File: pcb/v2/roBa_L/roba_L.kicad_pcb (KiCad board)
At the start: 2 copper layers, 123.9 x 94.5 mm, 56 parts, among them J1 Conn_01x01-Connector_Generic, J2 Conn_01x01-Connector_Generic, J3 Conn_01x01-Connector_Generic, J4 Conn_01x01-Connector_Generic, J5 Conn_01x01-Connector_Generic, J6 Conn_01x01-Connector_Generic, J7 Conn_01x01-Connector_Generic, SW1 SW_PUSH, SW10 SW_PUSH, SW11 SW_PUSH, SW12 SW_PUSH, SW13 SW_PUSH, SW14 SW_PUSH, SW15 SW_PUSH, SW16 SW_PUSH, SW17 SW_PUSH, SW18 SW_PUSH, SW19 SW_PUSH, SW2 SW_PUSH, SW20 SW_PUSH, SW21 RotaryEncoder_Switch, SW22 SW_PUSH, SW23 SW_PUSH, SW24 SW_SPDT, SW3 SW_PUSH, SW4 SW_PUSH, SW5 SW_PUSH, SW6 SW_PUSH, SW7 SW_PUSH, SW8 SW_PUSH, SW9 SW_PUSH

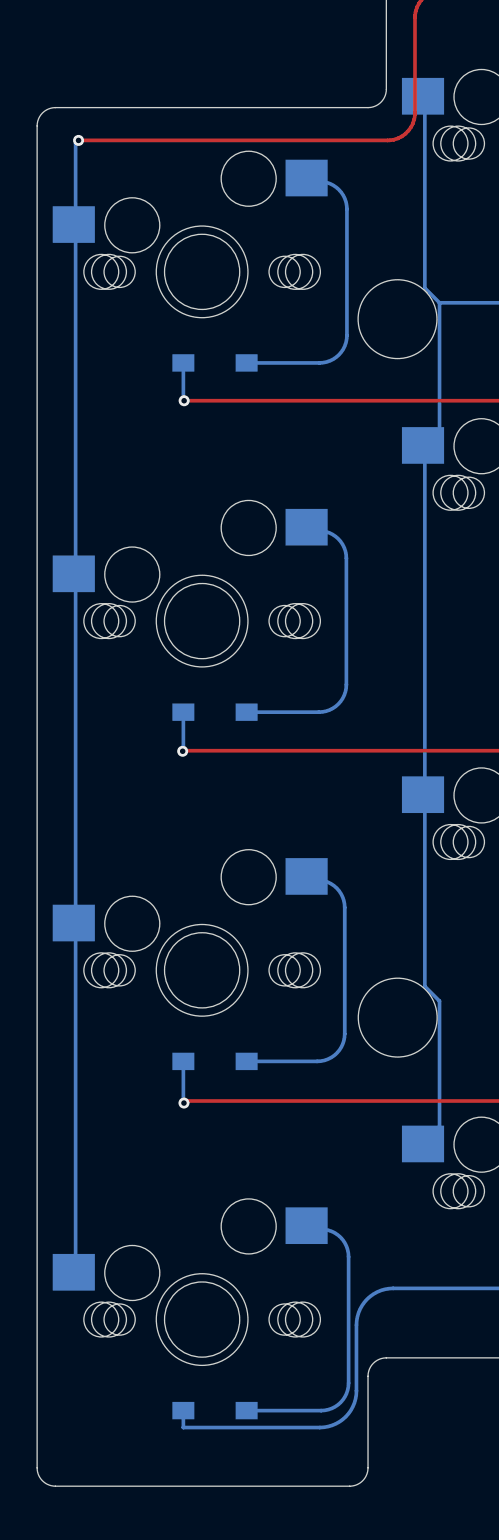
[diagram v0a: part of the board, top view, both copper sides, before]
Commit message: change partial switch
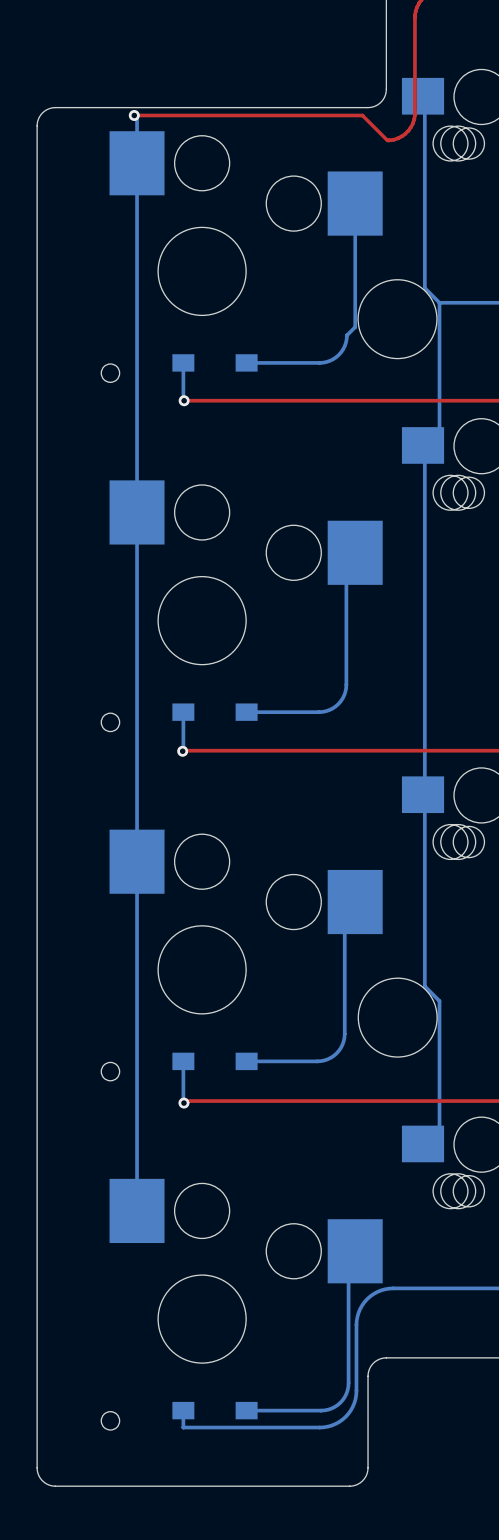
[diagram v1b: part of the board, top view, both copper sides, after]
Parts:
- SW1, SW2, SW3, SW4: footprint roBa:SW_MX -> ChocV2_Hotswap:Choc_v2_Hotswap_1u_MXcompatible.pretty
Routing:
- net Col0: track 187.6 -> 183.0 mm
- net Net-(D4-A): track 16.2 -> 13.3 mm
- net Net-(D2-A): track 16.0 -> 13.1 mm
- net Net-(D3-A): track 15.8 -> 13.0 mm
- net Net-(D1-A): track 16.1 -> 13.6 mm

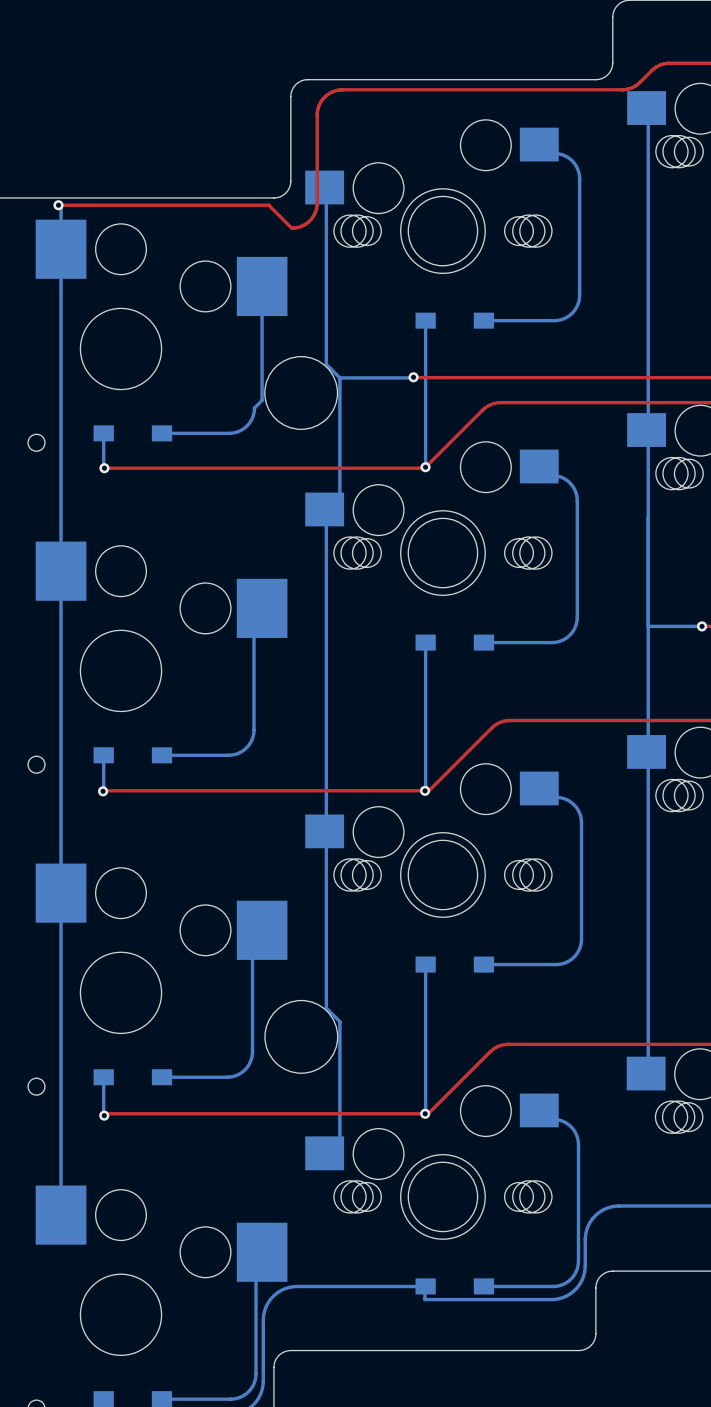
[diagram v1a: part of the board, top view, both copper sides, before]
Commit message: Lの二列目ok
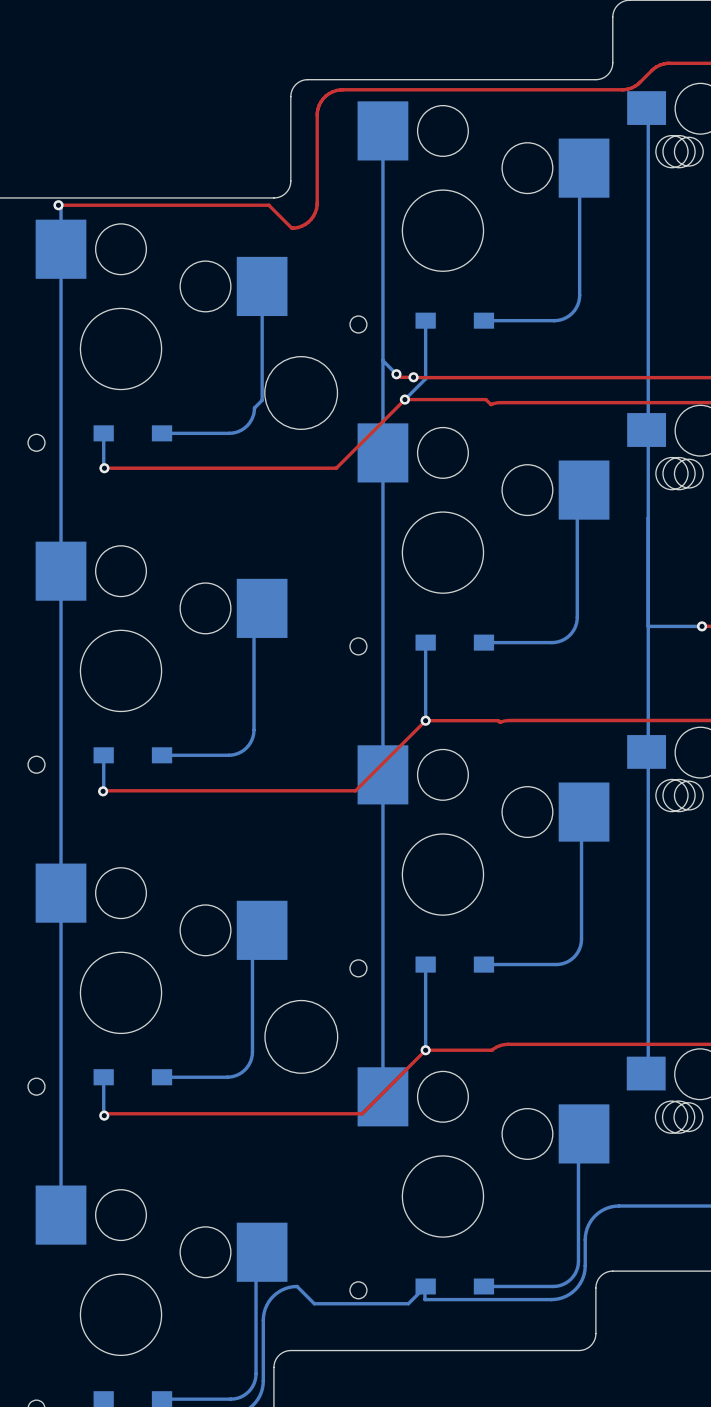
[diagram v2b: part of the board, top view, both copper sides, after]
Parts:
- SW5, SW6, SW7, SW8: footprint roBa:SW_MX -> ChocV2_Hotswap:Choc_v2_Hotswap_1u_MXcompatible.pretty
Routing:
- net Row1: track 154.8 -> 150.7 mm
- net Row2: track 177.2 -> 173.5 mm
- net Row0: track 122.6 -> 119.4 mm
- net Net-(D7-A): track 16.7 -> 13.5 mm
- net Net-(D5-A): track 16.4 -> 13.4 mm
- net Net-(D8-A): track 16.3 -> 13.3 mm
- net Net-(D6-A): track 16.2 -> 13.2 mm
- net Col1: track 158.8 -> 155.9 mm, vias 1 -> 2
- net Row3: track 201.8 -> 202.6 mm

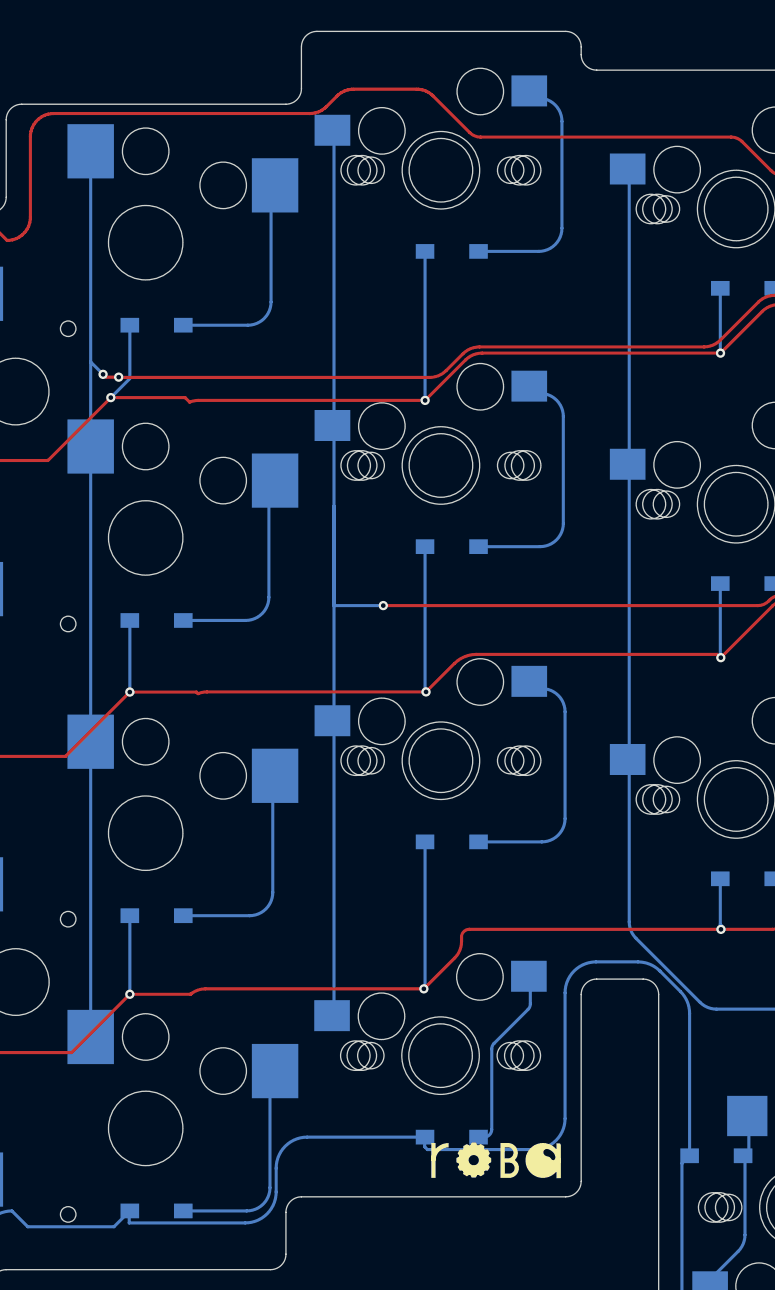
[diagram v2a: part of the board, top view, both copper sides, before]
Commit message: Lの三列目ok
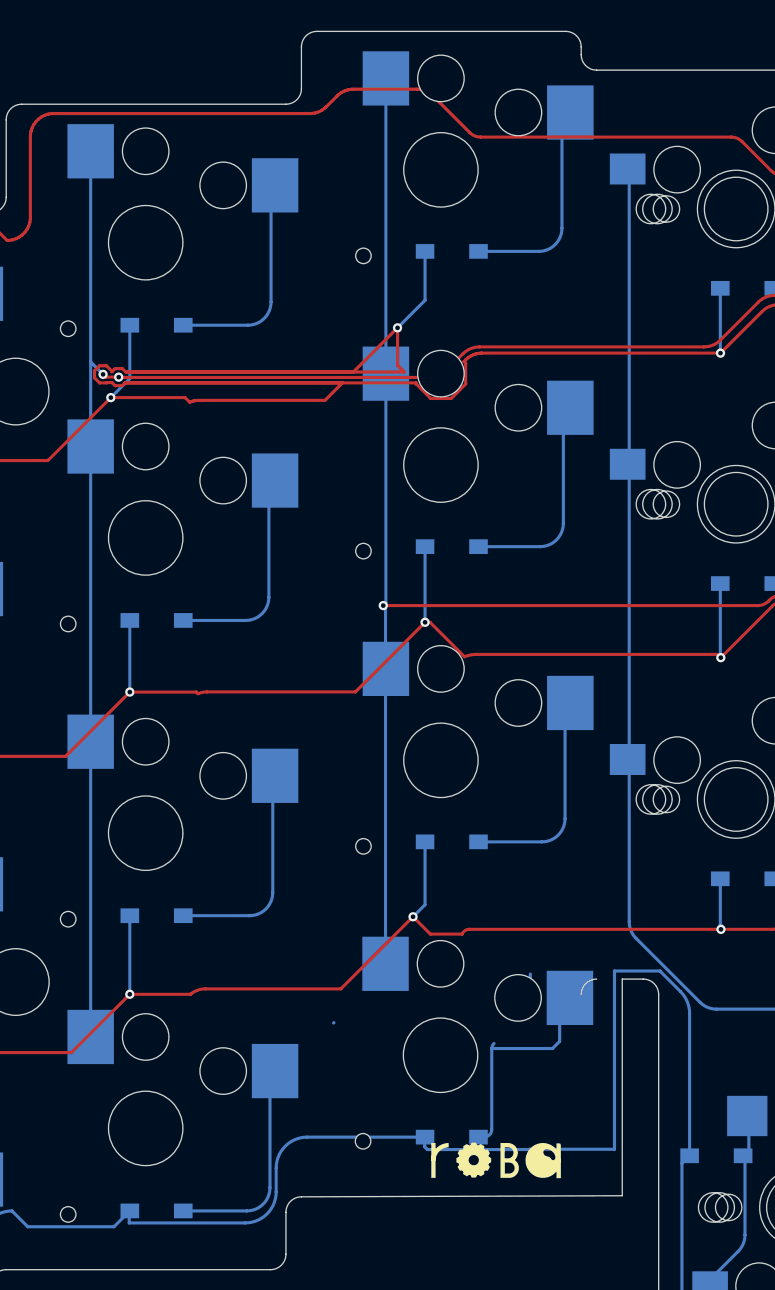
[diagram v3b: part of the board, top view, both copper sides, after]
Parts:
- SW10, SW11, SW12, SW9: footprint roBa:SW_MX -> ChocV2_Hotswap:Choc_v2_Hotswap_1u_MXcompatible.pretty
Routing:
- net Row0: track 119.4 -> 190.3 mm
- net Col2: track 148.6 -> 138.2 mm
- net Net-(D12-A): track 12.3 -> 16.6 mm
- net Row2: track 173.5 -> 169.5 mm
- net Net-(D11-A): track 16.3 -> 13.3 mm
- net Net-(D10-A): track 16.1 -> 13.2 mm
- net Net-(D9-A): track 15.9 -> 13.1 mm
- net Row1: track 150.7 -> 148.1 mm
- net Row3: track 202.6 -> 204.1 mm
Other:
- outline, holes or cut-outs redrawn
